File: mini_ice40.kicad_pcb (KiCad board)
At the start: 2 copper layers, 4 parts

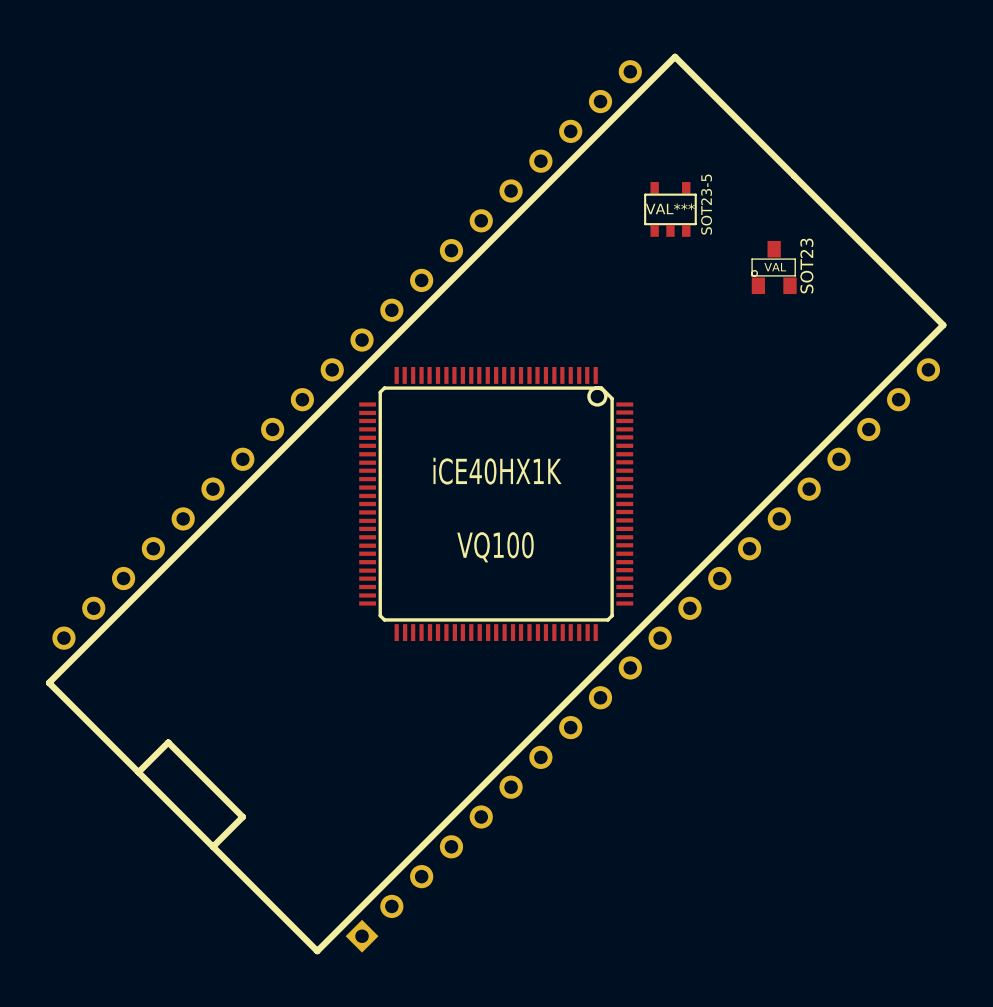
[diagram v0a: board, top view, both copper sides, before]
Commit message: ** Laid out PCB
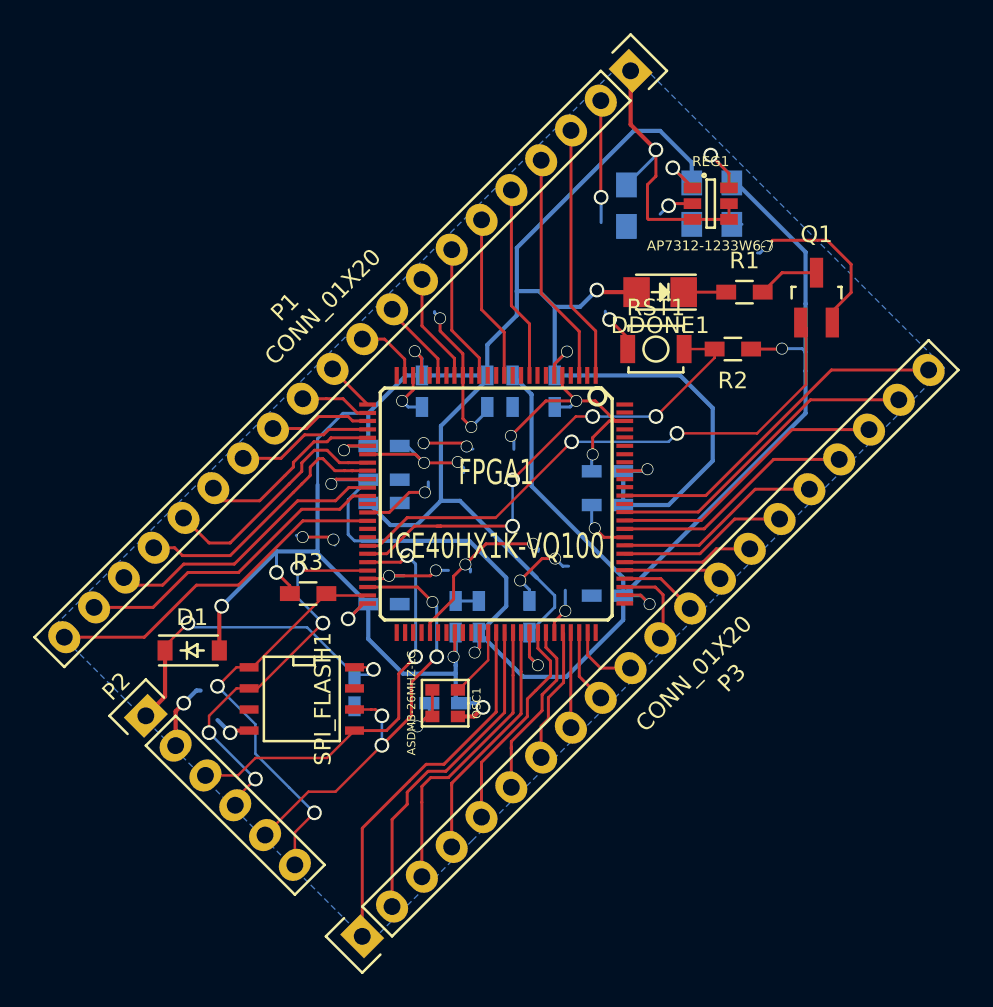
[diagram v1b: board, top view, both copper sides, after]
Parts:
- removed ?: , DIP-40__1000
- removed SOT23: VAL, SOT23
- removed SOT23-5: VAL***, SOT23-5
- removed iCE40HX1K: VQ100, VQFP100
- added C1: 1u, Capacitors_SMD:C_0805_HandSoldering, B.Cu at (101.3, 33.5)
- added C10: 0u1, Capacitors_SMD:C_0603_HandSoldering, B.Cu at (93.0, 44.7)
- added C11: 0u1, Capacitors_SMD:C_0603_HandSoldering, B.Cu at (91.1, 58.3)
- added C12: 0u1, Capacitors_SMD:C_0603_HandSoldering, B.Cu at (89.0, 44.7)
- added C13: 0u1, Capacitors_SMD:C_0603_HandSoldering, B.Cu at (100.2, 49.5)
- added C14: 0u1, Capacitors_SMD:C_0603_HandSoldering, B.Cu at (97.0, 44.7)
- added C15: 0u1, Capacitors_SMD:C_0603_HandSoldering, B.Cu at (86.7, 48.0)
- added C16: 0u1, Capacitors_SMD:C_0603_HandSoldering, B.Cu at (86.7, 50.0)
- added C17: 0u1, Capacitors_SMD:C_0603_HandSoldering, B.Cu at (94.5, 44.7)
- added C18: 0u1, Capacitors_SMD:C_0603_HandSoldering, B.Cu at (100.2, 57.0)
- added C19: 0u1, Capacitors_SMD:C_0603_HandSoldering, B.Cu at (92.5, 58.3)
- added C2: 1u, Capacitors_SMD:C_0805_HandSoldering, B.Cu at (105.3, 33.4)
- added C3: 1u, Capacitors_SMD:C_0805_HandSoldering, B.Cu at (107.7, 33.4)
- added C4: 0u1, Capacitors_SMD:C_0603_HandSoldering, B.Cu at (85.0, 62.7)
- added C5: 0u1, Capacitors_SMD:C_0603_HandSoldering, B.Cu at (90.4, 63.5)
- added C6: 0u1, Capacitors_SMD:C_0603_HandSoldering, B.Cu at (86.7, 57.5)
- added C7: 0u1, Capacitors_SMD:C_0603_HandSoldering, B.Cu at (100.2, 51.6)
- added C8: 0u1, Capacitors_SMD:C_0603_HandSoldering, B.Cu at (86.7, 51.4)
- added C9: 0u1, Capacitors_SMD:C_0603_HandSoldering, B.Cu at (95.5, 58.3)
- added D1: 1N4448WQ-7-F, Diodes_SMD:SOD-123, F.Cu at (75.2, 60.3)
- added DDONE1: SML-LX1206GC-TR1, LEDs:LED_1206, F.Cu at (103.4, 38.7)
- added FPGA1: ICE40HX1K-VQ100, mini_ice40:VQFP100, F.Cu at (93.5, 51.5)
- added OSC1: ASDMB-26MHZ-LC, mini_ice40:2MMx2MM5, F.Cu at (90.4, 63.5)
- added P1: CONN_01X20, Pin_Headers:Pin_Header_Straight_1x20, F.Cu at (101.6, 25.4)
- added P2: CONN_01X04, Pin_Headers:Pin_Header_Straight_1x06, F.Cu at (72.4, 64.3)
- added P3: CONN_01X20, Pin_Headers:Pin_Header_Straight_1x20, F.Cu at (85.4, 77.5)
- added Q1: 2N7002LT1G, TO_SOT_Packages_SMD:SOT-23_Handsoldering, F.Cu at (112.8, 39.1)
- added R1: 330, Resistors_SMD:R_0603_HandSoldering, F.Cu at (108.5, 38.7)
- added R2: 10K, Resistors_SMD:R_0603_HandSoldering, F.Cu at (107.8, 42.2)
- added R3: 10K, Resistors_SMD:R_0603_HandSoldering, F.Cu at (82.2, 56.9)
- added REG1: AP7312-1233W6-7, TO_SOT_Packages_SMD:SOT-23-6, F.Cu at (106.4, 33.4)
- added RST1: SW_PUSH, Buttons_Switches_SMD:SW_SPST_B3U-1000P, F.Cu at (103.1, 42.2)
- added SPI_FLASH1: AT25SF041-SSHD-B, SMD_Packages:SOIC-8-N, F.Cu at (81.8, 63.2)
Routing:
- net +3V3: track 0.00 -> 163.9 mm, vias 0 -> 12
- net GND: track 0.00 -> 106.9 mm, vias 0 -> 24
- net +1V2: track 0.00 -> 97.5 mm, vias 0 -> 5
- net Net-(FPGA1-Pad43): track 0.00 -> 34.3 mm, vias 0 -> 2
- net Net-(FPGA1-Pad44): track 0.00 -> 30.1 mm, vias 0 -> 4
- net Net-(FPGA1-Pad48): track 0.00 -> 27.6 mm, vias 0 -> 4
- net Net-(FPGA1-Pad45): track 0.00 -> 26.1 mm, vias 0 -> 2
- net Net-(FPGA1-Pad49): track 0.00 -> 25.0 mm, vias 0 -> 2
- net Net-(FPGA1-Pad46): track 0.00 -> 24.4 mm, vias 0 -> 4
- net Net-(FPGA1-Pad63): track 0.00 -> 23.1 mm
- net Net-(FPGA1-Pad89): track 0.00 -> 21.4 mm
- net Net-(FPGA1-Pad40): track 0.00 -> 21.2 mm
- net Net-(C4-Pad1): track 0.00 -> 20.4 mm, vias 0 -> 2
- net Net-(FPGA1-Pad64): track 0.00 -> 19.9 mm
- net Net-(FPGA1-Pad87): track 0.00 -> 19.3 mm
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- added copper zone on B.Cu, net GND
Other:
- net class Default: clearance 0.254 -> 0.2; trace_width 0.254 -> 0.18; via_dia 0.889 -> 0.72
- net class Thick added: clearance 0.2, trace_width 0.254, via_dia 0.72, via_drill 0.635
- rule trace_clearance: 0.254 -> 0.2
- rule trace_min: 0.254 -> 0.15
- rule via_min_size: 0.889 -> 0.72
